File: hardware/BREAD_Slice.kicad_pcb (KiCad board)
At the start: 2 copper layers, 70 x 100 mm, 15 parts, among them J1 Conn_01x10_Female

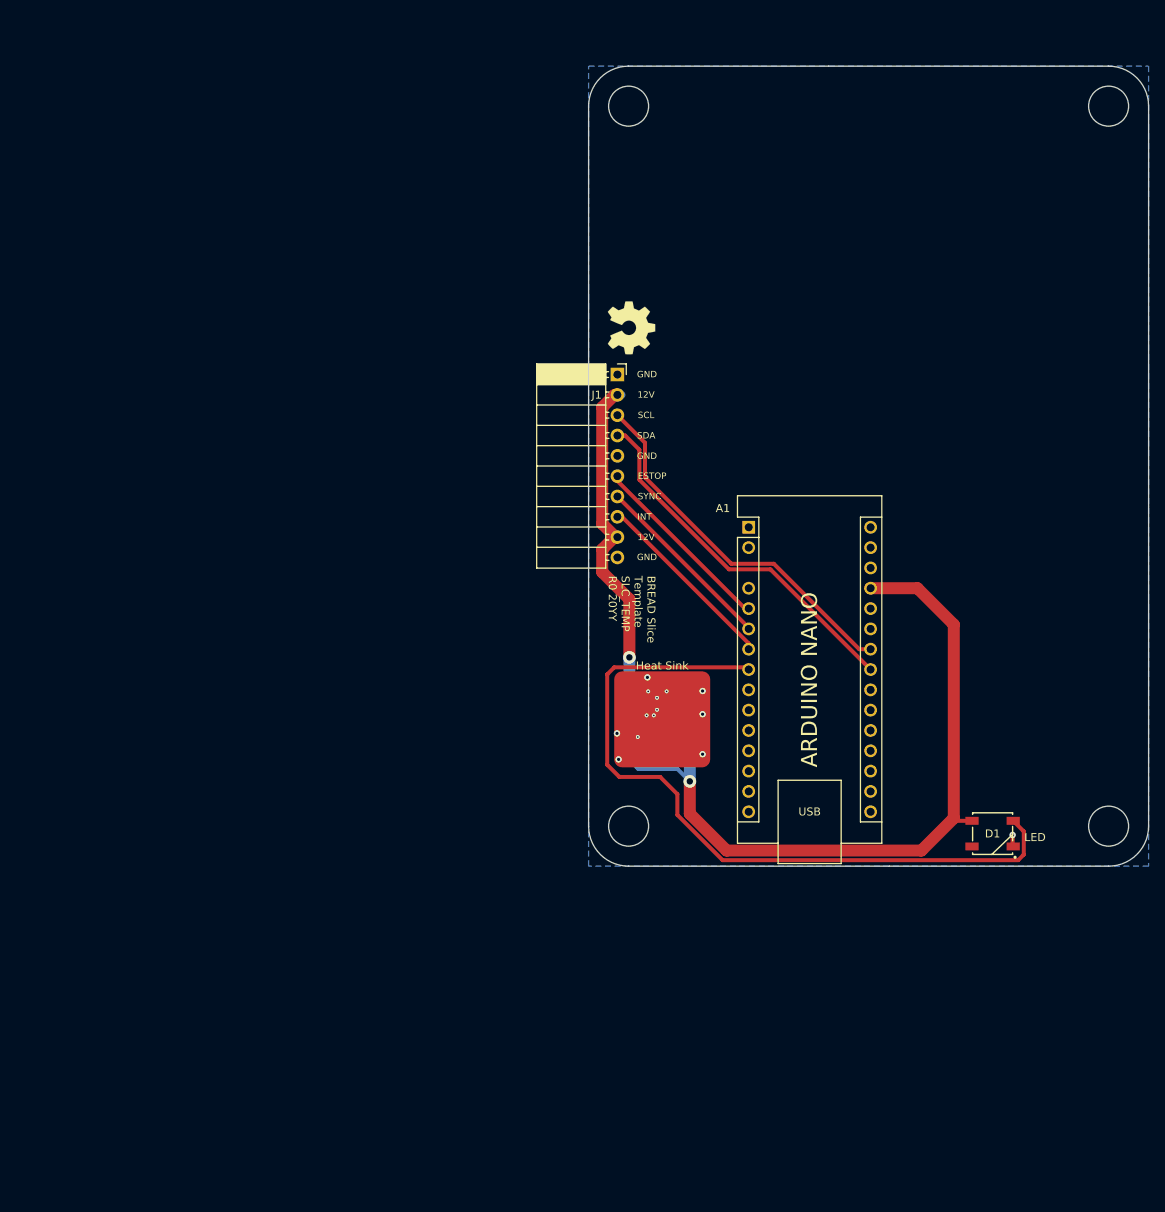
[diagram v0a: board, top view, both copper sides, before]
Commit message: completed schematic and board
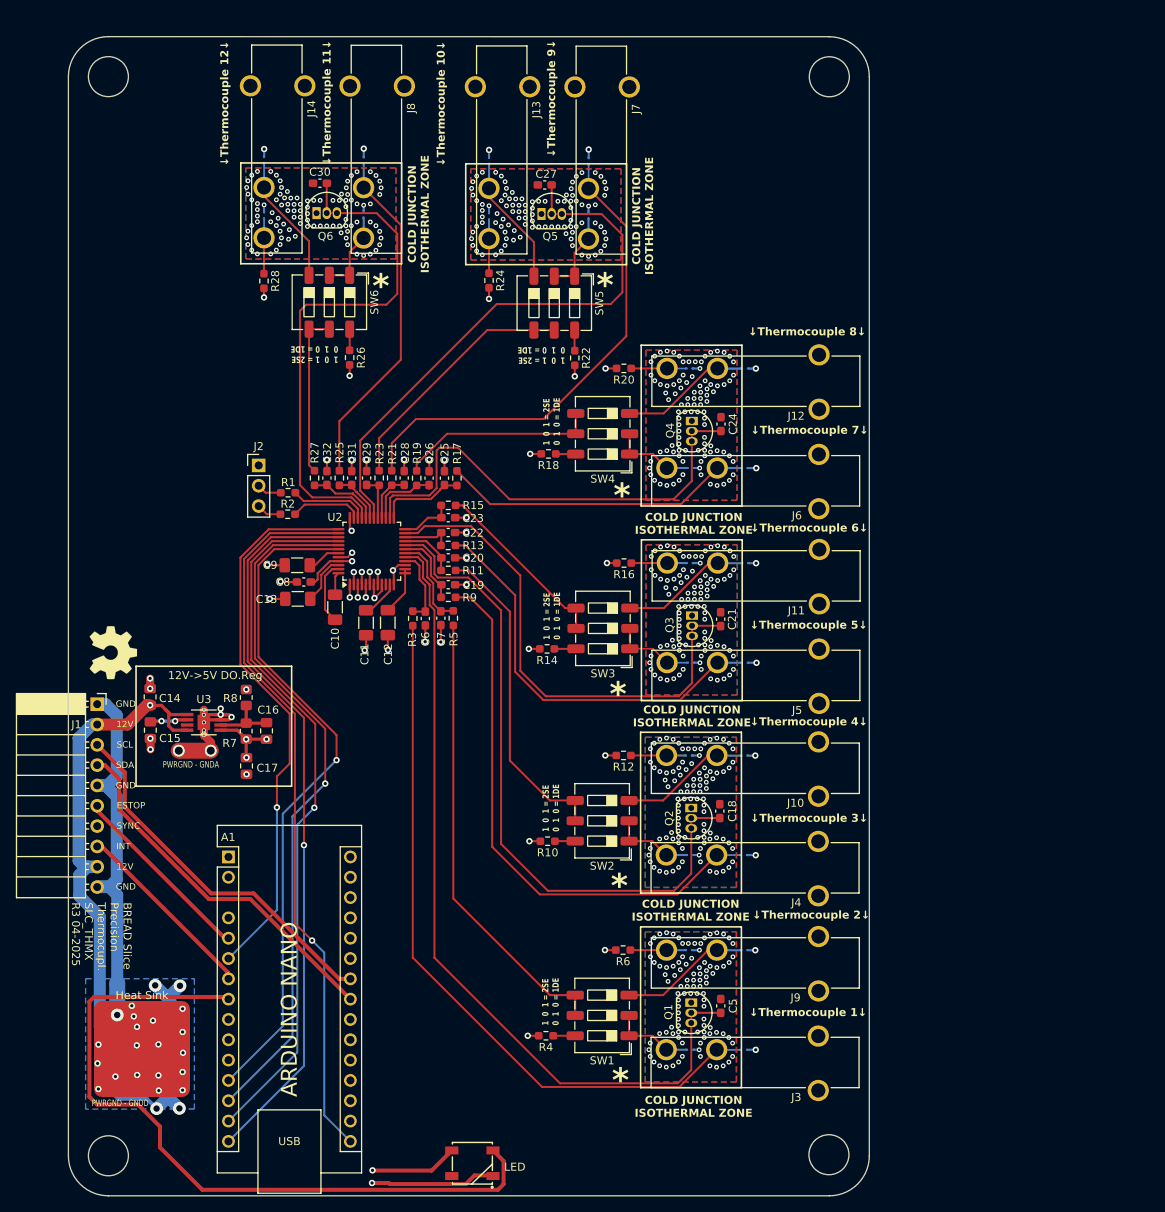
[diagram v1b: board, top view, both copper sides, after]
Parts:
- added C10: 10u X7R, Capacitor_SMD:C_1206_3216Metric_Pad1.33x1.80mm_HandSolder, F.Cu at (90.9, 107.4)
- added C11: 0.1u X7R, Capacitor_SMD:C_1206_3216Metric_Pad1.33x1.80mm_HandSolder, F.Cu at (94.8, 109.4)
- added C12: 1u X7R, Capacitor_SMD:C_1206_3216Metric_Pad1.33x1.80mm_HandSolder, F.Cu at (97.5, 109.4)
- added C13: 10u X5R, Capacitor_SMD:C_1206_3216Metric_Pad1.33x1.80mm_HandSolder, F.Cu at (86.2, 106.4)
- added C14: 10u, Capacitor_SMD:C_0805_2012Metric_Pad1.18x1.45mm_HandSolder, F.Cu at (67.8, 118.6)
- added C15: 10n, Capacitor_SMD:C_0805_2012Metric_Pad1.18x1.45mm_HandSolder, F.Cu at (67.8, 122.8)
- added C16: 10n, Capacitor_SMD:C_0805_2012Metric_Pad1.18x1.45mm_HandSolder, F.Cu at (82.3, 122.9)
- added C17: 10u, Capacitor_SMD:C_0805_2012Metric_Pad1.18x1.45mm_HandSolder, F.Cu at (79.8, 127.3)
- added C18: 0.01u, Capacitor_SMD:C_0603_1608Metric_Pad1.08x0.95mm_HandSolder, F.Cu at (139.0, 132.9)
- added C19: 0.1u, Capacitor_SMD:C_0603_1608Metric_Pad1.08x0.95mm_HandSolder, F.Cu at (105.1, 104.6)
- added C20: 0.1u, Capacitor_SMD:C_0603_1608Metric_Pad1.08x0.95mm_HandSolder, F.Cu at (105.1, 101.3)
- added C21: 0.01u, Capacitor_SMD:C_0603_1608Metric_Pad1.08x0.95mm_HandSolder, F.Cu at (139.1, 108.9)
- added C22: 0.1u, Capacitor_SMD:C_0603_1608Metric_Pad1.08x0.95mm_HandSolder, F.Cu at (105.0, 98.1)
- added C23: 0.1u, Capacitor_SMD:C_0603_1608Metric_Pad1.08x0.95mm_HandSolder, F.Cu at (105.1, 96.2)
- added C24: 0.01u, Capacitor_SMD:C_0603_1608Metric_Pad1.08x0.95mm_HandSolder, F.Cu at (139.2, 84.5)
- added C25: 0.1u, Capacitor_SMD:C_0603_1608Metric_Pad1.08x0.95mm_HandSolder, F.Cu at (104.6, 91.3)
- added C26: 0.1u, Capacitor_SMD:C_0603_1608Metric_Pad1.08x0.95mm_HandSolder, F.Cu at (102.7, 91.3)
- added C27: 0.01u, Capacitor_SMD:C_0603_1608Metric_Pad1.08x0.95mm_HandSolder, F.Cu at (117.1, 54.6)
- added C28: 0.1u, Capacitor_SMD:C_0603_1608Metric_Pad1.08x0.95mm_HandSolder, F.Cu at (99.5, 91.3)
- added C29: 0.1u, Capacitor_SMD:C_0603_1608Metric_Pad1.08x0.95mm_HandSolder, F.Cu at (94.8, 91.3)
- added C30: 0.01u, Capacitor_SMD:C_0603_1608Metric_Pad1.08x0.95mm_HandSolder, F.Cu at (89.0, 54.4)
- added C31: 0.1u, Capacitor_SMD:C_0603_1608Metric_Pad1.08x0.95mm_HandSolder, F.Cu at (93.0, 91.3)
- added C32: 0.1u, Capacitor_SMD:C_0603_1608Metric_Pad1.08x0.95mm_HandSolder, F.Cu at (89.9, 91.3)
- added C5: 0.01u, Capacitor_SMD:C_0603_1608Metric_Pad1.08x0.95mm_HandSolder, F.Cu at (139.1, 157.3)
- added C6: 0.1u, Capacitor_SMD:C_0603_1608Metric_Pad1.08x0.95mm_HandSolder, F.Cu at (102.2, 108.8)
- added C7: 0.1u, Capacitor_SMD:C_0603_1608Metric_Pad1.08x0.95mm_HandSolder, F.Cu at (104.1, 108.8)
- added C8: 0.1u X7R, Capacitor_SMD:C_0603_1608Metric_Pad1.08x0.95mm_HandSolder, F.Cu at (87.0, 104.3)
- added C9: 10u X7R, Capacitor_SMD:C_1206_3216Metric_Pad1.33x1.80mm_HandSolder, F.Cu at (86.2, 102.2)
- added D10: DF2S6.8MFS_L3M, Diode_SMD:D_SOD-923, B.Cu at (142.1, 114.4)
- added D11: DF2S6.8MFS_L3M, Diode_SMD:D_SOD-923, B.Cu at (135.4, 114.4)
- added D12: DF2S6.8MFS_L3M, Diode_SMD:D_SOD-923, B.Cu at (142.2, 101.9)
- added D13: DF2S6.8MFS_L3M, Diode_SMD:D_SOD-923, B.Cu at (135.2, 101.9)
- added D14: DF2S6.8MFS_L3M, Diode_SMD:D_SOD-923, B.Cu at (142.1, 90.0)
- added D15: DF2S6.8MFS_L3M, Diode_SMD:D_SOD-923, B.Cu at (135.3, 90.0)
- added D16: DF2S6.8MFS_L3M, Diode_SMD:D_SOD-923, B.Cu at (142.1, 77.6)
- added D17: DF2S6.8MFS_L3M, Diode_SMD:D_SOD-923, B.Cu at (135.2, 77.6)
- added D18: DF2S6.8MFS_L3M, Diode_SMD:D_SOD-923, B.Cu at (122.6, 51.7)
- added D19: DF2S6.8MFS_L3M, Diode_SMD:D_SOD-923, B.Cu at (122.6, 58.4)
- added D2: DF2S6.8MFS_L3M, Diode_SMD:D_SOD-923, B.Cu at (142.0, 162.8)
- added D20: DF2S6.8MFS_L3M, Diode_SMD:D_SOD-923, B.Cu at (110.2, 51.6)
- added D21: DF2S6.8MFS_L3M, Diode_SMD:D_SOD-923, B.Cu at (110.2, 58.6)
- added D22: DF2S6.8MFS_L3M, Diode_SMD:D_SOD-923, B.Cu at (94.5, 51.6)
- added D23: DF2S6.8MFS_L3M, Diode_SMD:D_SOD-923, B.Cu at (94.5, 58.3)
- added D24: DF2S6.8MFS_L3M, Diode_SMD:D_SOD-923, B.Cu at (82.0, 51.5)
- added D25: DF2S6.8MFS_L3M, Diode_SMD:D_SOD-923, B.Cu at (82.0, 58.5)
- added D3: DF2S6.8MFS_L3M, Diode_SMD:D_SOD-923, B.Cu at (135.3, 162.7)
- added D4: DF2S6.8MFS_L3M, Diode_SMD:D_SOD-923, B.Cu at (142.1, 150.3)
- added D5: DF2S6.8MFS_L3M, Diode_SMD:D_SOD-923, B.Cu at (135.1, 150.3)
- added D6: DF2S6.8MFS_L3M, Diode_SMD:D_SOD-923, B.Cu at (142.0, 138.4)
- added D7: DF2S6.8MFS_L3M, Diode_SMD:D_SOD-923, B.Cu at (135.3, 138.4)
- added D8: DF2S6.8MFS_L3M, Diode_SMD:D_SOD-923, B.Cu at (142.1, 126.0)
- added D9: DF2S6.8MFS_L3M, Diode_SMD:D_SOD-923, B.Cu at (135.1, 126.0)
- added J10: PCC-SMP-V-K, kml-custom:OMEGA_PCC-SMP-V-K, F.Cu at (132.3, 126.0)
- added J11: PCC-SMP-V-K, kml-custom:OMEGA_PCC-SMP-V-K, F.Cu at (132.4, 101.9)
- added J12: PCC-SMP-V-K, kml-custom:OMEGA_PCC-SMP-V-K, F.Cu at (132.4, 77.6)
- added J13: PCC-SMP-V-K, kml-custom:OMEGA_PCC-SMP-V-K, F.Cu at (110.1, 61.4)
- added J14: PCC-SMP-V-K, kml-custom:OMEGA_PCC-SMP-V-K, F.Cu at (82.0, 61.3)
- added J2: Conn_01x03_Pin, Connector_PinHeader_2.54mm:PinHeader_1x03_P2.54mm_Vertical, F.Cu at (81.4, 89.7)
- added J3: PCC-SMP-V-K, kml-custom:OMEGA_PCC-SMP-V-K, F.Cu at (132.3, 162.7)
- added J4: PCC-SMP-V-K, kml-custom:OMEGA_PCC-SMP-V-K, F.Cu at (132.3, 138.4)
- added J5: PCC-SMP-V-K, kml-custom:OMEGA_PCC-SMP-V-K, F.Cu at (132.4, 114.4)
- added J6: PCC-SMP-V-K, kml-custom:OMEGA_PCC-SMP-V-K, F.Cu at (132.4, 90.0)
- added J7: PCC-SMP-V-K, kml-custom:OMEGA_PCC-SMP-V-K, F.Cu at (122.6, 61.4)
- added J8: PCC-SMP-V-K, kml-custom:OMEGA_PCC-SMP-V-K, F.Cu at (94.5, 61.3)
- added J9: PCC-SMP-V-K, kml-custom:OMEGA_PCC-SMP-V-K, F.Cu at (132.3, 150.3)
- added NT1: NetTie_2, NetTie:NetTie-2_SMD_Pad2.0mm, B.Cu at (63.7, 156.4)
- added NT2: NetTie_2, NetTie:NetTie-2_SMD_Pad2.0mm, F.Cu at (73.4, 125.4)
- added Q1: 2N3904, Package_TO_SOT_THT:TO-92_Inline, F.Cu at (135.4, 156.9)
- added Q2: 2N3904, Package_TO_SOT_THT:TO-92_Inline, F.Cu at (135.4, 132.5)
- added Q3: 2N3904, Package_TO_SOT_THT:TO-92_Inline, F.Cu at (135.5, 108.5)
- added Q4: 2N3904, Package_TO_SOT_THT:TO-92_Inline, F.Cu at (135.5, 84.2)
- added Q5: 2N3904, Package_TO_SOT_THT:TO-92_Inline, F.Cu at (116.7, 58.3)
- added Q6: 2N3904, Package_TO_SOT_THT:TO-92_Inline, F.Cu at (88.6, 58.2)
- added R1: 1k, Resistor_SMD:R_0603_1608Metric_Pad0.98x0.95mm_HandSolder, F.Cu at (85.0, 93.1)
- added R10: 1k, Resistor_SMD:R_0603_1608Metric_Pad0.98x0.95mm_HandSolder, F.Cu at (117.5, 136.7)
- added R11: 1k, Resistor_SMD:R_0603_1608Metric_Pad0.98x0.95mm_HandSolder, F.Cu at (105.1, 102.8)
- added R12: 1k, Resistor_SMD:R_0603_1608Metric_Pad0.98x0.95mm_HandSolder, F.Cu at (127.0, 126.0)
- added R13: 1k, Resistor_SMD:R_0603_1608Metric_Pad0.98x0.95mm_HandSolder, F.Cu at (105.0, 99.7)
- added R14: 1k, Resistor_SMD:R_0603_1608Metric_Pad0.98x0.95mm_HandSolder, F.Cu at (117.4, 112.6)
- added R15: 1k, Resistor_SMD:R_0603_1608Metric_Pad0.98x0.95mm_HandSolder, F.Cu at (105.1, 94.7)
- added R16: 1k, Resistor_SMD:R_0603_1608Metric_Pad0.98x0.95mm_HandSolder, F.Cu at (127.0, 101.9)
- added R17: 1k, Resistor_SMD:R_0603_1608Metric_Pad0.98x0.95mm_HandSolder, F.Cu at (106.1, 91.3)
- added R18: 1k, Resistor_SMD:R_0603_1608Metric_Pad0.98x0.95mm_HandSolder, F.Cu at (117.6, 88.3)
- added R19: 1k, Resistor_SMD:R_0603_1608Metric_Pad0.98x0.95mm_HandSolder, F.Cu at (101.1, 91.3)
- added R2: 1k, Resistor_SMD:R_0603_1608Metric_Pad0.98x0.95mm_HandSolder, F.Cu at (85.0, 95.8)
- added R20: 1k, Resistor_SMD:R_0603_1608Metric_Pad0.98x0.95mm_HandSolder, F.Cu at (127.0, 77.6)
- added R21: 1k, Resistor_SMD:R_0603_1608Metric_Pad0.98x0.95mm_HandSolder, F.Cu at (98.0, 91.3)
- added R22: 1k, Resistor_SMD:R_0603_1608Metric_Pad0.98x0.95mm_HandSolder, F.Cu at (120.9, 76.3)
- added R23: 1k, Resistor_SMD:R_0603_1608Metric_Pad0.98x0.95mm_HandSolder, F.Cu at (96.4, 91.3)
- added R24: 1k, Resistor_SMD:R_0603_1608Metric_Pad0.98x0.95mm_HandSolder, F.Cu at (110.2, 66.6)
- added R25: 1k, Resistor_SMD:R_0603_1608Metric_Pad0.98x0.95mm_HandSolder, F.Cu at (91.4, 91.3)
- added R26: 1k, Resistor_SMD:R_0603_1608Metric_Pad0.98x0.95mm_HandSolder, F.Cu at (92.7, 76.2)
- added R27: 1k, Resistor_SMD:R_0603_1608Metric_Pad0.98x0.95mm_HandSolder, F.Cu at (88.3, 91.3)
- added R28: 1k, Resistor_SMD:R_0603_1608Metric_Pad0.98x0.95mm_HandSolder, F.Cu at (82.0, 66.7)
- added R3: 1k, Resistor_SMD:R_0603_1608Metric_Pad0.98x0.95mm_HandSolder, F.Cu at (100.6, 108.8)
- added R4: 1k, Resistor_SMD:R_0603_1608Metric_Pad0.98x0.95mm_HandSolder, F.Cu at (117.3, 161.0)
- added R5: 1k, Resistor_SMD:R_0603_1608Metric_Pad0.98x0.95mm_HandSolder, F.Cu at (105.7, 108.8)
- added R6: 1k, Resistor_SMD:R_0603_1608Metric_Pad0.98x0.95mm_HandSolder, F.Cu at (126.9, 150.3)
- added R7: 99, Resistor_SMD:R_0805_2012Metric_Pad1.20x1.40mm_HandSolder, F.Cu at (79.8, 122.9)
- added R8: 99, Resistor_SMD:R_0805_2012Metric_Pad1.20x1.40mm_HandSolder, F.Cu at (79.8, 118.7)
- added R9: 1k, Resistor_SMD:R_0603_1608Metric_Pad0.98x0.95mm_HandSolder, F.Cu at (105.1, 106.2)
- added SW1: SW_DIP_x03, Button_Switch_SMD:SW_DIP_SPSTx03_Slide_6.7x9.18mm_W6.73mm_P2.54mm_LowProfile_JPin, F.Cu at (124.3, 158.5)
- added SW2: SW_DIP_x03, Button_Switch_SMD:SW_DIP_SPSTx03_Slide_6.7x9.18mm_W6.73mm_P2.54mm_LowProfile_JPin, F.Cu at (124.3, 134.1)
- added SW3: SW_DIP_x03, Button_Switch_SMD:SW_DIP_SPSTx03_Slide_6.7x9.18mm_W6.73mm_P2.54mm_LowProfile_JPin, F.Cu at (124.4, 110.1)
- added SW4: SW_DIP_x03, Button_Switch_SMD:SW_DIP_SPSTx03_Slide_6.7x9.18mm_W6.73mm_P2.54mm_LowProfile_JPin, F.Cu at (124.4, 85.7)
- added SW5: SW_DIP_x03, Button_Switch_SMD:SW_DIP_SPSTx03_Slide_6.7x9.18mm_W6.73mm_P2.54mm_LowProfile_JPin, F.Cu at (118.3, 69.4)
- added SW6: SW_DIP_x03, Button_Switch_SMD:SW_DIP_SPSTx03_Slide_6.7x9.18mm_W6.73mm_P2.54mm_LowProfile_JPin, F.Cu at (90.2, 69.3)
- added U2: LTC2983, Package_QFP:LQFP-48_7x7mm_P0.5mm, F.Cu at (95.5, 100.4)
- added U3: TPS7A4901DGNR, kml-custom:DGN8_1P89X1P57, F.Cu at (74.5, 121.8)
- HS1: footprint KML-Custom:Thermal Pad -> kml-custom:Thermal Pad
- U1: value ~ -> AP63205
- moved A1 77.0 mm to (77.6, 138.6)
- moved C1 77.0 mm to (63.8, 160.7)
- moved C2 77.0 mm to (66.1, 167.5)
- moved D1 77.0 mm to (108.1, 176.9)
- moved J1 77.0 mm to (61.2, 119.6)
- moved L1 77.0 mm to (68.8, 164.0)
- moved U1 77.0 mm to (63.7, 164.0)
- moved C3 77.0 mm to (68.8, 160.7)
- moved HS1 77.0 mm to (66.8, 162.7)
- moved H2 77.0 mm to (62.6, 176.0)
- moved C4 77.0 mm to (68.8, 157.6)
- moved Logo1 76.4 mm to (63.2, 113.1)
- moved H1 65.1 mm to (62.6, 41.1)
- moved H4 53.9 mm to (152.6, 175.9)
- moved H3 35.1 mm to (152.7, 41.1)
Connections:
- net /E_STOP renamed /ESTOP
- A1 pad 10: /D7 -> unconnected-(A1-D7-Pad10)
- A1 pad 11: /D8 -> unconnected-(A1-D8-Pad11)
- A1 pad 12: /D9 -> /RESET
- A1 pad 13: /D10 -> /SS
- A1 pad 14: /D11 -> /MOSI
- A1 pad 15: /D12 -> /MISO
- A1 pad 16: /D13 -> /SCK
- A1 pad 18: /AREF -> unconnected-(A1-AREF-Pad18)
- A1 pad 19: /A0 -> unconnected-(A1-A0-Pad19)
- A1 pad 20: /A1 -> unconnected-(A1-A1-Pad20)
- A1 pad 21: /A2 -> unconnected-(A1-A2-Pad21)
- A1 pad 22: /A3 -> unconnected-(A1-A3-Pad22)
- A1 pad 25: /A6 -> unconnected-(A1-A6-Pad25)
- A1 pad 26: /A7 -> unconnected-(A1-A7-Pad26)
- A1 pad 28: /RESET -> unconnected-(A1-~{RESET}-Pad28)
- A1 pad 9: /D6 -> unconnected-(A1-D6-Pad9)
- J1 pad 1: GND -> GNDPWR
- J1 pad 10: GND -> GNDPWR
- J1 pad 5: GND -> GNDPWR
- J1 pad 7: /INT -> unconnected-(J1-Pin_7-Pad7)
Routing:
- net /CH2: track 0.00 -> 102.6 mm
- net GNDA: track 0.00 -> 96.3 mm, vias 0 -> 647
- net /MISO: track 0.00 -> 92.0 mm, vias 0 -> 1
- net /SCK: track 0.00 -> 91.4 mm, vias 0 -> 1
- net /Dual Selectable SE-DE Thermocouple CJC Input1/TC_1+: track 0.00 -> 91.1 mm
- net /MOSI: track 0.00 -> 89.7 mm, vias 0 -> 1
- net /SS: track 0.00 -> 87.2 mm, vias 0 -> 1
- net /RESET: track 0.00 -> 84.9 mm, vias 0 -> 1
- net /CH5: track 0.00 -> 83.4 mm
- net /CH15: track 0.00 -> 71.5 mm
- net /Dual Selectable SE-DE Thermocouple CJC Input2/TC_1+: track 0.00 -> 69.7 mm
- net /CH18: track 0.00 -> 66.1 mm
- net /CH8: track 0.00 -> 63.5 mm
- net +5V: track 104.2 -> 42.4 mm, vias 1 -> 5
- net /Dual Selectable SE-DE Thermocouple CJC Input5/TC_1+: track 0.00 -> 61.7 mm
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- added copper zone on In2.Cu, net +12V
- added copper zone on In2.Cu, net +5V
- added copper zone on In2.Cu, net +5VA
- added copper zone on In1.Cu, net GND
- added copper zone on B.Cu, net GNDA
- added copper zone on F.Cu, net GNDA
- added copper zone on In1.Cu, net GNDA
- added copper zone on In1.Cu, net GNDPWR
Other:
- board size 70 x 100 mm -> 100.1 x 144.9 mm
- copper layers 2 -> 4
- board text added: "*"
- board text added: "1 0 1 = 2SE 0 1 0 = 1DE"
- board text added: "12V->5V DO.Reg"
- board text added: "12V->5V Sw.Reg"
- board text added: "BREAD Slice Precision Thermocupl. SLC_THMX R3 04-2025"
- board text added: "COLD JUNCTION ISOTHERMAL ZONE"
- board text added: "L1 (Top): - Template digital components (Nano, RGB LED) and I²C signals - use minimal ground pours. L2 (Inner 1): - Solid ground plane - split into an upper {dblquote}gndpwr{dblquote} zone (handling 12V returns) and a lower digital ground zone, connected only at the regulator - these can be resized to accommadate additional planes - i.e. decreasing 12V/GNDPWR planes to connector edge and creating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"
- board text added: "PWRGND - GNDA"
- board text added: "PWRGND - GNDD"
- board text added: "↓Thermocouple 10↓"
- board text added: "↓Thermocouple 11↓"
- board text added: "↓Thermocouple 12↓"
- board text added: "↓Thermocouple 1↓"
- board text added: "↓Thermocouple 2↓"
- board text added: "↓Thermocouple 3↓"
- board text added: "↓Thermocouple 4↓"
- board text added: "↓Thermocouple 5↓"
- board text added: "↓Thermocouple 6↓"
- board text added: "↓Thermocouple 7↓"
- board text added: "↓Thermocouple 8↓"
- board text added: "↓Thermocouple 9↓"
- board text removed: "12V->5V Reg"
- board text removed: "5V I2C Connector"
- board text removed: "BREAD Slice Template SLC_TEMP R0 20YY"
